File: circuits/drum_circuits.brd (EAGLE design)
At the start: 79.9 x 51.2 mm, 39 parts, among them U1 OPA344, U2 ATMEGA328P_TQFP, U3 ADMP401

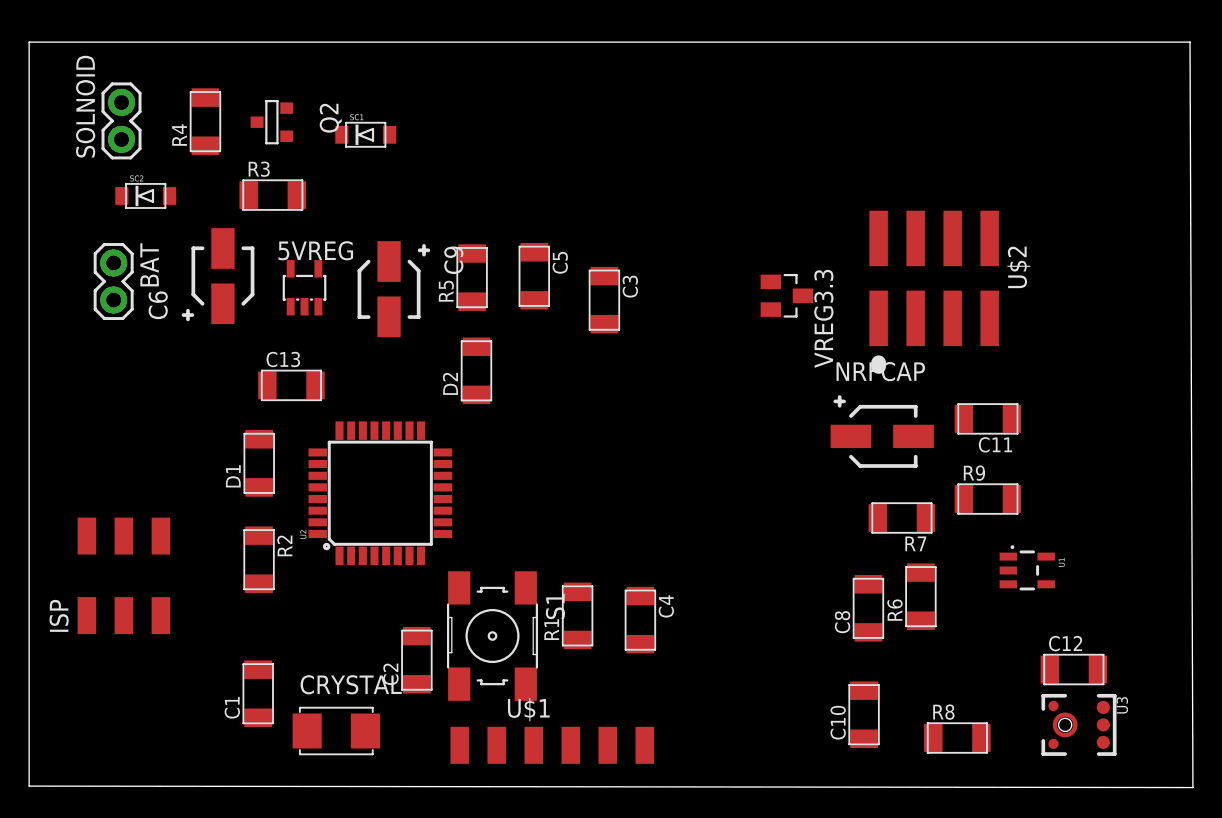
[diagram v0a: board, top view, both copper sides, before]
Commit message: overwriting board & schematic from 5d2ad6c18a5f5ec5e8afae34b5d28b62efabe567
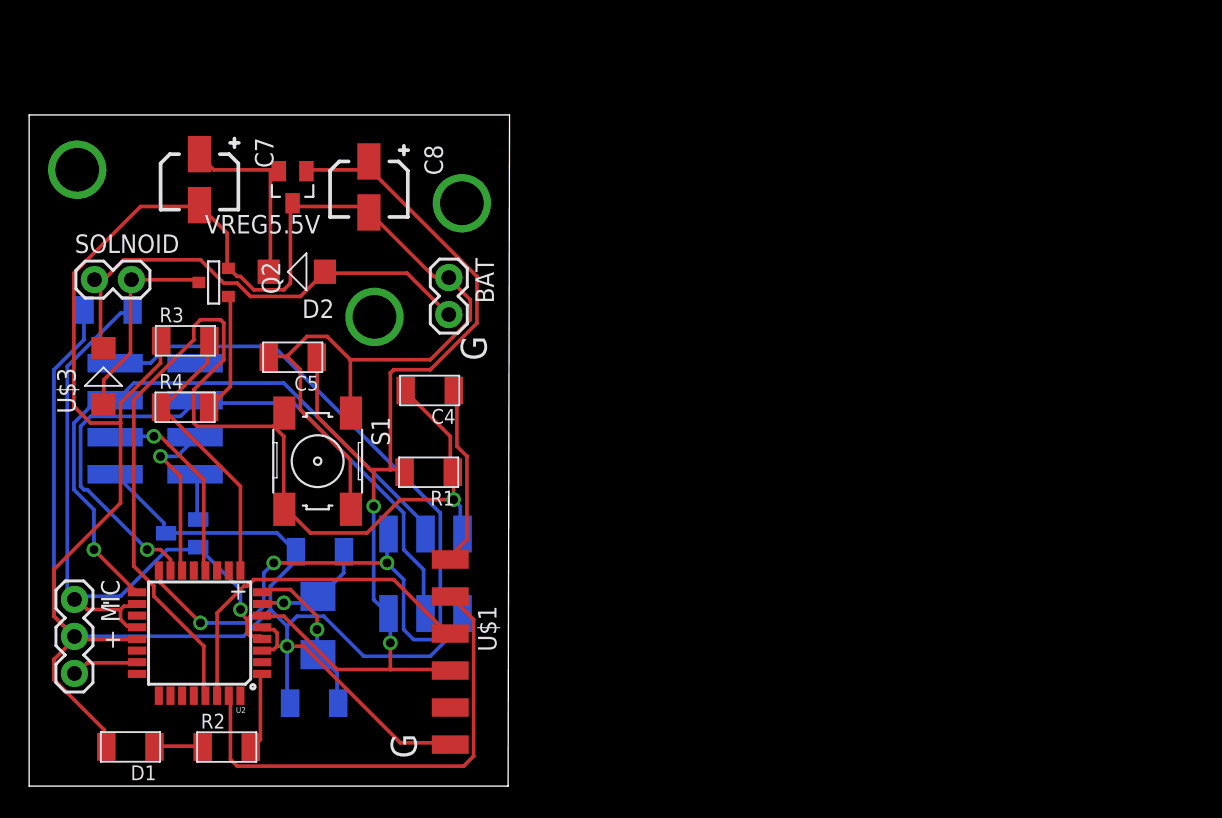
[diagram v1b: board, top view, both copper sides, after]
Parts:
- removed 5VREG: MIC5225-5v, adafruit:SOT23-5L
- removed C10: 1uF, fab:C1206FAB
- removed C11: 100pF, fab:C1206FAB
- removed C12, C13: 0.1uF, fab:C1206FAB
- removed C6, C9: 10uF, talkingdrums:PANASONIC-CAP-SMD-B
- removed NRFCAP: 33uF, talkingdrums:PANASONIC-CAP-SMD-C
- removed R5: 500, fab:R1206FAB
- removed R6: 1.5K, fab:R1206FAB
- removed R7, R8: 10k, fab:R1206FAB
- removed R9: 100k, fab:R1206FAB
- removed SC1, SC2: (no value), adafruit:SOD-123FL
- removed U1: OPA344, SparkFun-AnalogIC:SOT23-5
- removed U3: ADMP401, SparkFun-Sensors:ADMP401
- added C7: 10uF, talkingdrums:PANASONIC-CAP-SMD-B
- added MIC: (no value), SparkFun-Connectors:1X03
- added U$3: RECTIFIER, talkingdrums:RECTIFIER
- added VREG5.5V: 7805, fab:SOT23
- C8: value 4.7uF -> 10uF; device fab:C1206FAB -> talkingdrums:PANASONIC-CAP-SMD-B
- D2: value LEDFAB1206 -> RECTIFIER; device fab:LED1206FAB -> talkingdrums:RECTIFIER
- moved U$2 53.5 mm to (5.80, 21.4), flipped to the bottom, turned to 0 degrees
- moved C8 46.0 mm to (23.2, 42.9), turned to 180 degrees
- moved VREG3.3 44.6 mm to (10.4, 17.4), flipped to the bottom
- moved C3 34.0 mm to (5.35, 32.7), flipped to the bottom, turned to 0 degrees
- moved BAT 23.0 mm to (28.7, 34.9)
- moved C4 21.4 mm to (27.4, 27.1), turned to 180 degrees
- moved D1 21.4 mm to (6.85, 2.69), turned to 180 degrees
- moved ISP 20.7 mm to (27.1, 14.8), flipped to the bottom, turned to 270 degrees
- moved R4 19.6 mm to (10.6, 26.0), turned to 0 degrees
- moved C5 17.5 mm to (18.0, 29.4), turned to 180 degrees
- moved S1 17.0 mm to (19.7, 22.3)
- moved U2 15.7 mm to (11.6, 10.5), turned to 180 degrees
- moved R1 14.2 mm to (27.3, 21.5), turned to 180 degrees
- moved R2 13.1 mm to (13.5, 2.68), turned to 0 degrees
- moved D2 12.4 mm to (20.2, 35.3), turned to 180 degrees
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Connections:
- net N$10 renamed LED
- net N$11 renamed GATE
- removed net N$6: D2.1, R5.2
- removed net N$7: C8.2, R6.2
- removed net N$8: C10.2, C11.1, R6.1, R7.2, R8.2, R9.2, U1.3, U1.4
- removed net N$9: C13.2, U2.20
- removed net VBUS: ISP.2, SC1.A, U$1.3
- net 3.3V: no longer C12.2, R7.1, U1.5, U3.5
- net 5V: now also C8.POS, ISP.2, MIC.1, U$1.3, U2.20, VREG5.5V.1; no longer 5VREG.5, C9.POS, R5.1, SC1.C
- net DRAIN: now also U$3.1; no longer SC2.A
- net GND: now also C7.NEG, C8.NEG, MIC.2, VREG5.5V.3; no longer 5VREG.2, C10.1, C12.1, C13.1, C6.NEG, C9.NEG, D2.2, R8.1, U$1.2, U1.2, U3.2, U3.4, U3.6
- net MIC: now also MIC.3; no longer C11.2, R9.1, U1.1
- net N$4: now also C7.POS, D2.2, VREG5.5V.2; no longer C8.1, U3.1
- net VCC: now also D2.1, U$3.2; no longer 5VREG.1, 5VREG.3, C6.POS, SC2.C
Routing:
- net GND: track 0.00 -> 223.6 mm, vias 0 -> 1
- net 5V: track 0.00 -> 121.8 mm, vias 0 -> 3
- net RST: track 0.00 -> 77.8 mm, vias 0 -> 1
- net MISO: track 0.00 -> 66.5 mm, vias 0 -> 3
- net MOSI: track 0.00 -> 46.9 mm, vias 0 -> 1
- net SCK: track 0.00 -> 43.4 mm, vias 0 -> 1
- net RX: track 0.00 -> 33.3 mm
- net VCC: track 0.00 -> 33.1 mm
- net TX: track 0.00 -> 24.1 mm
- net GATE_DO: track 0.00 -> 19.5 mm
- net DRAIN: track 0.00 -> 14.1 mm
- net CE: track 0.00 -> 13.6 mm, vias 0 -> 1
- net N$4: track 0.00 -> 13.0 mm
- net DTR: track 0.00 -> 12.5 mm
- net CSN: track 0.00 -> 11.4 mm, vias 0 -> 1
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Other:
- board size 79.9 x 51.2 mm -> 33 x 46.1 mm
- board text added: "+"
- board text added: "-"
- board text added: "G"
